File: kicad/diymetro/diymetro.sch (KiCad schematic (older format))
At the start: 45 parts, among them J1 Conn_02x08_Top_Bottom, J10 ReverseSwitch, J11 Conn_01x04, J12 +5V, J2 CLKGATE_Pots, J3 Gate_Pots, J4 CV_Pots, J5 CLKOUT, J6 GATEOUT, J7 CVOUT, J8 LEDs, J9 Conn_01x04, U1 74HC4051, U2 74HC4051, U3 74LS594, U4 74LS165

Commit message: Update schematic a bit.
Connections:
- net labels added: CLK165, SHLD
- net labels removed: CE, CP
- wire segments 155 -> 156
- no-connect marks 24 -> 23
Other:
- note added: "Wiring Notes:\n\n* Connect pots to +5V and GND. \n* Pot tapers to the CV + Gate connectors.\n* Pots are 10k.\n* Connect jacks to GND and connectors.\n* Connect switches to +5V and connectors.\n* LED cathodes to GND and LED connector.\n* Play with 74LS594 resistors to match your LEDs."
- moved on the sheet: J1, R12, R13, R14, R15, R16, R17, R18, R19

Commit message: Work on clock input.
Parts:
- added J13: CLOCK_INPUT, symbol Connector:AudioJack2_SwitchT
- added Q1: PN2222A, Package_TO_SOT_THT:TO-92_Inline, symbol Transistor_BJT:PN2222A
- added R20: 1M, Resistor_THT:R_Axial_DIN0207_L6.3mm_D2.5mm_P7.62mm_Horizontal, symbol Device:R
- added R21: 100K, Resistor_THT:R_Axial_DIN0207_L6.3mm_D2.5mm_P7.62mm_Horizontal, symbol Device:R
- added R22: 10K, Resistor_THT:R_Axial_DIN0207_L6.3mm_D2.5mm_P7.62mm_Horizontal, symbol Device:R
- J10: value ReverseSwitch -> MainSW
- J5: value CLKOUT -> GATEOUT
- J6: value GATEOUT -> CLKOUT
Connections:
- net labels added: CINSW, CLK_IN
- wire segments 156 -> 172
- no-connect marks 23 -> 21
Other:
- moved on the sheet: C1, C2, C3, C4, C5, D1, D2, J1, R1, R10, R11, R3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

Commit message: Update code and schematics for clock and reset input.
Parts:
- removed J10: MainSW, Connector_PinHeader_2.54mm:PinHeader_1x01_P2.54mm_Vertical, symbol Connector:Conn_01x01_Female
- added J10: MAINSW, Connector_PinHeader_2.54mm:PinHeader_1x01_P2.54mm_Vertical, symbol Connector_Generic:Conn_01x01
- added J14: RESET_INPUT, symbol Connector:AudioJack2_SwitchT
- added Q2: PN2222A, Package_TO_SOT_THT:TO-92_Inline, symbol Transistor_BJT:PN2222A
- added R23: 100K, Resistor_THT:R_Axial_DIN0207_L6.3mm_D2.5mm_P7.62mm_Horizontal, symbol Device:R
- added R24: 10K, Resistor_THT:R_Axial_DIN0207_L6.3mm_D2.5mm_P7.62mm_Horizontal, symbol Device:R
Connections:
- net labels added: RST_IN
- net labels removed: CLK165
- wire segments 172 -> 180
- no-connect marks 21 -> 22
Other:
- moved on the sheet: C1, C2, C3, C4, C5, C6, D1, D2, D3, J1, J13, Q1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

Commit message: New schematics and boards.
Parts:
- removed A1: Arduino_Nano_v3.x, Module:Arduino_Nano, symbol MCU_Module:Arduino_Nano_v3.x
- removed C1, C3: 220n, Capacitor_THT:C_Rect_L7.0mm_W3.5mm_P2.50mm_P5.00mm, symbol Device:C
- removed C2, C4: 100n, Capacitor_THT:C_Axial_L3.8mm_D2.6mm_P7.50mm_Horizontal, symbol Device:C
- removed D3: D, Diode_THT:D_DO-15_P10.16mm_Horizontal, symbol Device:D
- removed J1: Conn_02x08_Top_Bottom, Connector_PinHeader_2.54mm:PinHeader_2x08_P2.54mm_Vertical, symbol Connector_Generic:Conn_02x08_Odd_Even
- removed J10: MAINSW, Connector_PinHeader_2.54mm:PinHeader_1x01_P2.54mm_Vertical, symbol Connector_Generic:Conn_01x01
- removed J11, J9: Conn_01x04, Connector_PinHeader_2.54mm:PinHeader_1x04_P2.54mm_Vertical, symbol Connector_Generic:Conn_01x04
- removed J12: +5V, Connector_PinHeader_2.54mm:PinHeader_1x01_P2.54mm_Vertical, symbol Connector_Generic:Conn_01x01
- removed J13: CLOCK_INPUT, symbol Connector:AudioJack2_SwitchT
- removed J14: RESET_INPUT, symbol Connector:AudioJack2_SwitchT
- removed J2: CLKGATE_Pots, Connector_PinHeader_2.54mm:PinHeader_1x02_P2.54mm_Vertical, symbol Connector_Generic:Conn_01x02
- removed J3: Gate_Pots, Connector_PinHeader_2.54mm:PinHeader_1x08_P2.54mm_Vertical, symbol Connector_Generic:Conn_01x08
- removed J4: CV_Pots, Connector_PinHeader_2.54mm:PinHeader_1x08_P2.54mm_Vertical, symbol Connector_Generic:Conn_01x08
- removed J5: GATEOUT, Connector_PinHeader_2.54mm:PinHeader_1x01_P2.54mm_Vertical, symbol Connector_Generic:Conn_01x01
- removed J6: CLKOUT, Connector_PinHeader_2.54mm:PinHeader_1x01_P2.54mm_Vertical, symbol Connector_Generic:Conn_01x01
- removed J7: CVOUT, Connector_PinHeader_2.54mm:PinHeader_1x01_P2.54mm_Vertical, symbol Connector_Generic:Conn_01x01
- removed J8: LEDs, Connector_PinHeader_2.54mm:PinHeader_1x08_P2.54mm_Vertical, symbol Connector_Generic:Conn_01x08
- removed R10, R11, R8, R9: 220, Resistor_THT:R_Axial_DIN0207_L6.3mm_D2.5mm_P7.62mm_Horizontal, symbol Device:R
- removed R12, R13, R14, R15, R16, R17, R18, R19, R22, R24: 10K, Resistor_THT:R_Axial_DIN0207_L6.3mm_D2.5mm_P7.62mm_Horizontal, symbol Device:R
- removed R20: 1M, Resistor_THT:R_Axial_DIN0207_L6.3mm_D2.5mm_P7.62mm_Horizontal, symbol Device:R
- removed R21, R23: 100K, Resistor_THT:R_Axial_DIN0207_L6.3mm_D2.5mm_P7.62mm_Horizontal, symbol Device:R
- removed U1, U2: 74HC4051, Package_DIP:DIP-16_W7.62mm, symbol 74xx:74HC4051
- removed U3: 74LS594, Package_DIP:DIP-16_W7.62mm, symbol 74xx_IEEE:74LS594
- removed U4: 74LS165, Package_DIP:DIP-16_W7.62mm, symbol 74xx:74LS165
- added C7, C8: 100n, Capacitor_SMD:C_1206_3216Metric, symbol Device:C
- added D14: LED, LED_THT:LED_D3.0mm, symbol Device:LED
- added J1, J2, J3, J4, J6: AudioJack2_SwitchT, Connector_Audio:Jack_3.5mm_QingPu_WQP-PJ398SM_Vertical_CircularHoles, symbol Connector:AudioJack2_SwitchT
- added J5: Conn_02x08_Top_Bottom, Connector_IDC:IDC-Header_2x08_P2.54mm_Vertical, symbol Connector_Generic:Conn_02x08_Odd_Even
- added J7: ICSP, Connector_PinHeader_2.54mm:PinHeader_2x03_P2.54mm_Vertical, symbol Connector_Generic:Conn_02x03_Odd_Even
- added J8: SER, Connector_PinHeader_2.54mm:PinHeader_1x02_P2.54mm_Vertical, symbol Connector:Conn_01x02_Male
- added R45: 10k, Resistor_SMD:R_1206_3216Metric, symbol Device:R
- added R46: 1K, Resistor_SMD:R_1206_3216Metric, symbol Device:R
- added RV1, RV2: R_POT, Potentiometer_THT:Potentiometer_Alps_RK09K_Single_Vertical, symbol Device:R_POT
- added SW10: SW_Push, Button_Switch_THT:SW_PUSH_6mm, symbol Switch:SW_Push
- added U5: ATmega328P-PU, Package_DIP:DIP-28_W7.62mm, symbol MCU_Microchip_ATmega:ATmega328P-PU
- added Y1: Crystal, Crystal:Crystal_HC49-4H_Vertical, symbol Device:Crystal
- C5, C6: value 100n -> 22p; footprint Capacitor_THT:C_Axial_L3.8mm_D2.6mm_P7.50mm_Horizontal -> Capacitor_SMD:C_1206_3216Metric
- D1, D2: footprint Diode_THT:D_DO-15_P10.16mm_Horizontal -> Diode_SMD:D_1206_3216Metric
- Q1, Q2: footprint Package_TO_SOT_THT:TO-92_Inline -> Package_TO_SOT_SMD:SOT-23
- R1, R2, R3: footprint Resistor_THT:R_Axial_DIN0207_L6.3mm_D2.5mm_P7.62mm_Horizontal -> Resistor_SMD:R_1206_3216Metric
- R4, R7: value 220 -> 100K; footprint Resistor_THT:R_Axial_DIN0207_L6.3mm_D2.5mm_P7.62mm_Horizontal -> Resistor_SMD:R_1206_3216Metric
- R5: value 220 -> 10K; footprint Resistor_THT:R_Axial_DIN0207_L6.3mm_D2.5mm_P7.62mm_Horizontal -> Resistor_SMD:R_1206_3216Metric
- R6: value 220 -> 1M; footprint Resistor_THT:R_Axial_DIN0207_L6.3mm_D2.5mm_P7.62mm_Horizontal -> Resistor_SMD:R_1206_3216Metric
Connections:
- net labels added: AP_CLK_IN, AP_CLK_OUT, AP_GATE_OUT, AP_RST_IN, ICSP_MISO, ICSP_MOSI, ICSP_RST, ICSP_SCK, PIN_CLKPOT, PIN_CVOUT, PIN_GATEOUT, PIN_GATEPOT, RA, SA
- net labels removed: CLK_IN, QH, RST_IN, SHLD
- wire segments 180 -> 84
- no-connect marks 22 -> 14
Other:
- note removed: "Wiring Notes:\n\n* Connect pots to +5V and GND. \n* Pot tapers to the CV + Gate connectors.\n* Pots are 10k.\n* Connect jacks to GND and connectors.\n* Connect switches to +5V and connectors.\n* LED cathodes to GND and LED connector.\n* Play with 74LS594 resistors to match your LEDs."

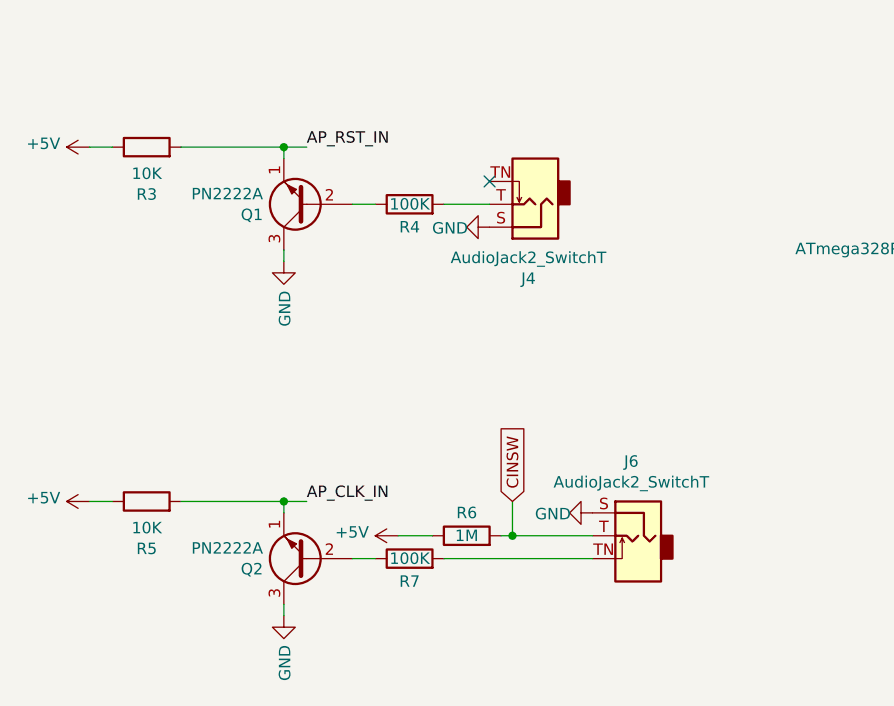
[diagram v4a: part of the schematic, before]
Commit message: Fix 74hc595 OE pin, Fix MBT2222A symbol + footprint, Fix clock-in jack connections.
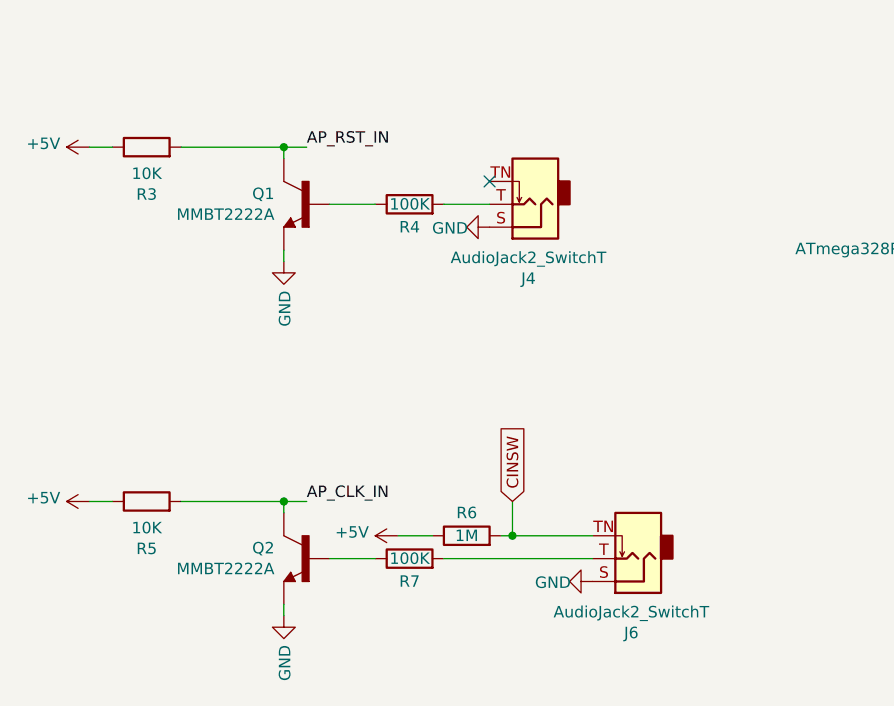
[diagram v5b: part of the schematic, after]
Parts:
- removed Q1, Q2: PN2222A, Package_TO_SOT_SMD:SOT-23, symbol Transistor_BJT:PN2222A
- added Q1, Q2: MMBT2222A, MMBT2222A:SOT23, symbol MMBT2222A:MMBT2222A
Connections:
- net AP_CLK_IN: now also Q2.3 (C)
- net AP_RST_IN: now also Q1.3 (C)
- net CINSW: now also J6.TN; no longer J6.T
- net GND: now also Q1.2 (E), Q2.2 (E)
- net at R7.1: now also Q2.1 (B)
- net at R7.2: now also J6.T; no longer J6.TN
- net at R4.1: now also Q1.1 (B)
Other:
- moved on the sheet: J6
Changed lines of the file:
@@
 	8500 3850 8550 3850
-$Comp
-L Transistor_BJT:PN2222A Q?
-U 1 1 5D188326
-P 2400 6050
-AR Path="/5CAA6291/5D188326" Ref="Q?"  Part="1"
-AR Path="/5D188326" Ref="Q2"  Part="1"
-F 0 "Q2" H 2591 6096 50  0000 L CNN
-F 1 "PN2222A" H 2591 6005 50  0000 L CNN
-F 2 "Package_TO_SOT_SMD:SOT-23" H 2600 5975 50  0001 L CIN
-F 3 "http://www.fairchildsemi.com/ds/PN/PN2222A.pdf" H 2400 6050 50  0001 L CNN
-	1    2400 6050
-	-1   0    0    1
-$EndComp
 $Comp
 L Device:R R?
@@
 	0    -1   -1   0
 $EndComp
-Wire Wire Line
-	2600 6050 2700 6050
 $Comp
 L power:GND #PWR?
@@
 Wire Wire Line
 	3250 5950 3300 5950
-Connection ~ 3300 5950
 Wire Wire Line
 	3300 5800 3300 5950
@@
 	2300 6300 2300 6250
 $Comp
-L Transistor_BJT:PN2222A Q?
-U 1 1 5D188368
-P 2400 4500
-AR Path="/5CAA6291/5D188368" Ref="Q?"  Part="1"
-AR Path="/5D188368" Ref="Q1"  Part="1"
-F 0 "Q1" H 2591 4546 50  0000 L CNN
-F 1 "PN2222A" H 2591 4455 50  0000 L CNN
-F 2 "Package_TO_SOT_SMD:SOT-23" H 2600 4425 50  0001 L CIN
-F 3 "http://www.fairchildsemi.com/ds/PN/PN2222A.pdf" H 2400 4500 50  0001 L CNN
-	1    2400 4500
-	-1   0    0    1
-$EndComp
-$Comp
 L Device:R R?
 U 1 1 5D18836F
@@
 	0    -1   -1   0
 $EndComp
-Wire Wire Line
-	2600 4500 2700 4500
 $Comp
 L power:GND #PWR?
@@
 L Connector:AudioJack2_SwitchT J?
 U 1 1 5D194F65
-P 3850 5950
+P 3850 6050
 AR Path="/5CA98B27/5D194F65" Ref="J?"  Part="1"
 AR Path="/5D194F65" Ref="J6"  Part="1"
-F 0 "J6" H 3880 6275 50  0000 C CNN
-F 1 "AudioJack2_SwitchT" H 3880 6184 50  0000 C CNN
-F 2 "Connector_Audio:Jack_3.5mm_QingPu_WQP-PJ398SM_Vertical_CircularHoles" H 3850 5950 50  0001 C CNN
-F 3 "~" H 3850 5950 50  0001 C CNN
-	1    3850 5950
-	-1   0    0    -1
+F 0 "J6" H 3880 6375 50  0000 C CNN
+F 1 "AudioJack2_SwitchT" H 3880 6284 50  0000 C CNN
+F 2 "Connector_Audio:Jack_3.5mm_QingPu_WQP-PJ398SM_Vertical_CircularHoles" H 3850 6050 50  0001 C CNN
+F 3 "~" H 3850 6050 50  0001 C CNN
+	1    3850 6050
+	-1   0    0    1
 $EndComp
 $Comp
@@
 Wire Wire Line
 	3000 6050 3650 6050
-Wire Wire Line
-	3300 5950 3650 5950
 $Comp
 L power:GND #PWR?
 U 1 1 5D1BFD84
-P 3650 5850
+P 3650 6150
 AR Path="/5CAA6291/5D1BFD84" Ref="#PWR?"  Part="1"
 AR Path="/5D1BFD84" Ref="#PWR031"  Part="1"
-F 0 "#PWR031" H 3650 5600 50  0001 C CNN
-F 1 "GND" V 3655 5677 50  0000 C CNN
-F 2 "" H 3650 5850 50  0001 C CNN
-F 3 "" H 3650 5850 50  0001 C CNN
-	1    3650 5850
+F 0 "#PWR031" H 3650 5900 50  0001 C CNN
+F 1 "GND" V 3655 5977 50  0000 C CNN
+F 2 "" H 3650 6150 50  0001 C CNN
+F 3 "" H 3650 6150 50  0001 C CNN
+	1    3650 6150
 	0    1    1    0
 $EndComp
@@
 	0    -1   -1   0
 $EndComp
+Wire Wire Line
+	2500 4500 2700 4500
+$Comp
+L MMBT2222A:MMBT2222A Q2
+U 1 1 5D860213
+P 2400 6050
+F 0 "Q2" H 2541 6096 50  0000 L CNN
+F 1 "MMBT2222A" H 2541 6005 50  0000 L CNN
+F 2 "MMBT2222A:SOT23" H 2400 6050 50  0001 L BNN
+F 3 "Unavailable" H 2400 6050 50  0001 L BNN
+F 4 "Fairchild Semiconductor" H 2400 6050 50  0001 L BNN "Field4"
+F 5 "MMBT2222 Series 40 V CE Breakdown 1 A NPN General Purpose Amplifier - SOT-23" H 2400 6050 50  0001 L BNN "Field5"
+F 6 "None" H 2400 6050 50  0001 L BNN "Field6"
+F 7 "SOT-23 Fairchild Semiconductor" H 2400 6050 50  0001 L BNN "Field7"
+F 8 "MMBT2222A." H 2400 6050 50  0001 L BNN "Field8"
+	1    2400 6050
+	-1   0    0    -1
+$EndComp
+Wire Wire Line
+	2500 6050 2700 6050
+$Comp
+L MMBT2222A:MMBT2222A Q1
+U 1 1 5D862FDE
+P 2400 4500
+F 0 "Q1" H 2541 4546 50  0000 L CNN
+F 1 "MMBT2222A" H 2541 4455 50  0000 L CNN
+F 2 "MMBT2222A:SOT23" H 2400 4500 50  0001 L BNN
+F 3 "Unavailable" H 2400 4500 50  0001 L BNN
+F 4 "Fairchild Semiconductor" H 2400 4500 50  0001 L BNN "Field4"
+F 5 "MMBT2222 Series 40 V CE Breakdown 1 A NPN General Purpose Amplifier - SOT-23" H 2400 4500 50  0001 L BNN "Field5"
+F 6 "None" H 2400 4500 50  0001 L BNN "Field6"
+F 7 "SOT-23 Fairchild Semiconductor" H 2400 4500 50  0001 L BNN "Field7"
+F 8 "MMBT2222A." H 2400 4500 50  0001 L BNN "Field8"
+	1    2400 4500
+	-1   0    0    -1
+$EndComp
+Connection ~ 3300 5950
+Wire Wire Line
+	3300 5950 3650 5950
 $EndSCHEMATC

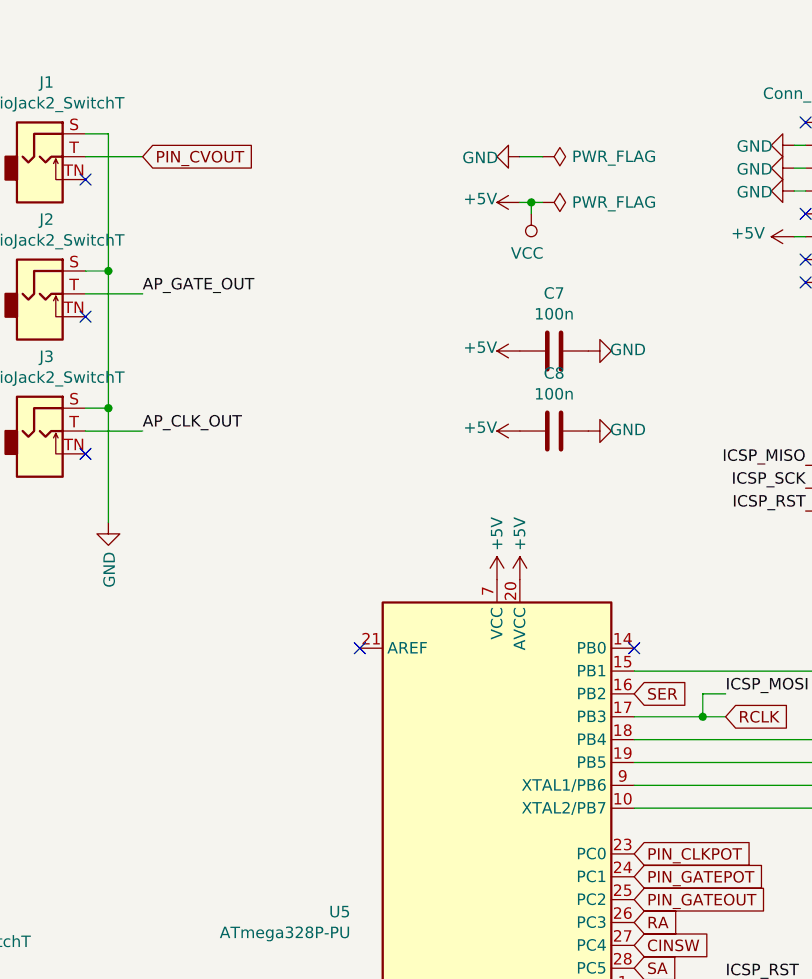
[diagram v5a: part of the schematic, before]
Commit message: Add missing C9
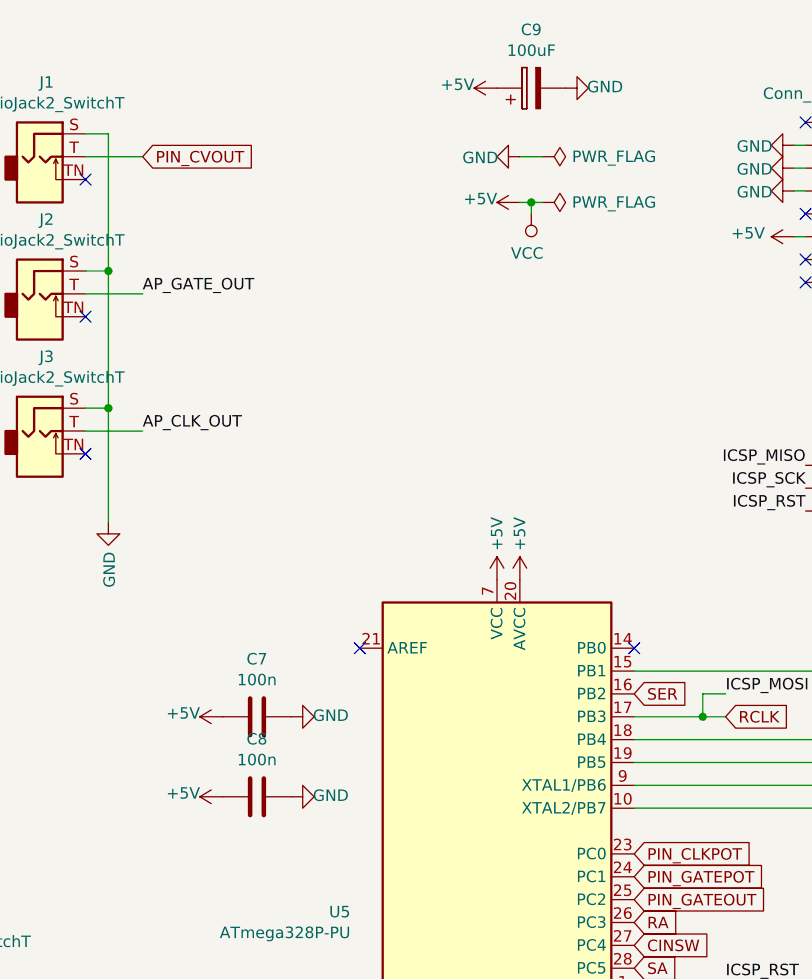
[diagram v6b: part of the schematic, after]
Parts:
- added C9: 100uF, symbol Device:CP
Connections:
- net +5V: now also C9.1
- net GND: now also C9.2
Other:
- moved on the sheet: C7, C8
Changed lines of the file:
@@
 L power:+5V #PWR?
 U 1 1 5D744A36
-P 5850 2150
+P 4550 3750
 AR Path="/5CAA6291/5D744A36" Ref="#PWR?"  Part="1"
 AR Path="/5D744A36" Ref="#PWR08"  Part="1"
-F 0 "#PWR08" H 5850 2000 50  0001 C CNN
-F 1 "+5V" V 5865 2323 50  0000 C CNN
-F 2 "" H 5850 2150 50  0001 C CNN
-F 3 "" H 5850 2150 50  0001 C CNN
-	1    5850 2150
+F 0 "#PWR08" H 4550 3600 50  0001 C CNN
+F 1 "+5V" V 4565 3923 50  0000 C CNN
+F 2 "" H 4550 3750 50  0001 C CNN
+F 3 "" H 4550 3750 50  0001 C CNN
+	1    4550 3750
 	0    -1   -1   0
 $EndComp
@@
 L Device:C C7
 U 1 1 5D744A7B
-P 6000 2150
-F 0 "C7" V 5748 2150 50  0000 C CNN
-F 1 "100n" V 5839 2150 50  0000 C CNN
-F 2 "Capacitor_SMD:C_1206_3216Metric" H 6038 2000 50  0001 C CNN
-F 3 "~" H 6000 2150 50  0001 C CNN
-	1    6000 2150
+P 4700 3750
+F 0 "C7" V 4448 3750 50  0000 C CNN
+F 1 "100n" V 4539 3750 50  0000 C CNN
+F 2 "Capacitor_SMD:C_1206_3216Metric" H 4738 3600 50  0001 C CNN
+F 3 "~" H 4700 3750 50  0001 C CNN
+	1    4700 3750
 	0    1    1    0
 $EndComp
@@
 L power:GND #PWR?
 U 1 1 5D744B09
-P 6150 2150
+P 4850 3750
 AR Path="/5CAA6291/5D744B09" Ref="#PWR?"  Part="1"
 AR Path="/5D744B09" Ref="#PWR015"  Part="1"
-F 0 "#PWR015" H 6150 1900 50  0001 C CNN
-F 1 "GND" V 6155 1977 50  0000 C CNN
-F 2 "" H 6150 2150 50  0001 C CNN
-F 3 "" H 6150 2150 50  0001 C CNN
-	1    6150 2150
+F 0 "#PWR015" H 4850 3500 50  0001 C CNN
+F 1 "GND" V 4855 3577 50  0000 C CNN
+F 2 "" H 4850 3750 50  0001 C CNN
+F 3 "" H 4850 3750 50  0001 C CNN
+	1    4850 3750
 	0    -1   -1   0
 $EndComp
@@
 L power:+5V #PWR?
 U 1 1 5D744CC7
-P 5850 2500
+P 4550 4100
 AR Path="/5CAA6291/5D744CC7" Ref="#PWR?"  Part="1"
 AR Path="/5D744CC7" Ref="#PWR029"  Part="1"
-F 0 "#PWR029" H 5850 2350 50  0001 C CNN
-F 1 "+5V" V 5865 2673 50  0000 C CNN
-F 2 "" H 5850 2500 50  0001 C CNN
-F 3 "" H 5850 2500 50  0001 C CNN
-	1    5850 2500
+F 0 "#PWR029" H 4550 3950 50  0001 C CNN
+F 1 "+5V" V 4565 4273 50  0000 C CNN
+F 2 "" H 4550 4100 50  0001 C CNN
+F 3 "" H 4550 4100 50  0001 C CNN
+	1    4550 4100
 	0    -1   -1   0
 $EndComp
@@
 L Device:C C8
 U 1 1 5D744CCD
-P 6000 2500
-F 0 "C8" V 5748 2500 50  0000 C CNN
-F 1 "100n" V 5839 2500 50  0000 C CNN
-F 2 "Capacitor_SMD:C_1206_3216Metric" H 6038 2350 50  0001 C CNN
-F 3 "~" H 6000 2500 50  0001 C CNN
-	1    6000 2500
+P 4700 4100
+F 0 "C8" V 4448 4100 50  0000 C CNN
+F 1 "100n" V 4539 4100 50  0000 C CNN
+F 2 "Capacitor_SMD:C_1206_3216Metric" H 4738 3950 50  0001 C CNN
+F 3 "~" H 4700 4100 50  0001 C CNN
+	1    4700 4100
 	0    1    1    0
 $EndComp
@@
 L power:GND #PWR?
 U 1 1 5D744CD4
-P 6150 2500
+P 4850 4100
 AR Path="/5CAA6291/5D744CD4" Ref="#PWR?"  Part="1"
 AR Path="/5D744CD4" Ref="#PWR034"  Part="1"
-F 0 "#PWR034" H 6150 2250 50  0001 C CNN
-F 1 "GND" V 6155 2327 50  0000 C CNN
-F 2 "" H 6150 2500 50  0001 C CNN
-F 3 "" H 6150 2500 50  0001 C CNN
-	1    6150 2500
+F 0 "#PWR034" H 4850 3850 50  0001 C CNN
+F 1 "GND" V 4855 3927 50  0000 C CNN
+F 2 "" H 4850 4100 50  0001 C CNN
+F 3 "" H 4850 4100 50  0001 C CNN
+	1    4850 4100
 	0    -1   -1   0
 $EndComp
@@
 Wire Wire Line
 	3300 5950 3650 5950
+$Comp
+L Device:CP C9
+U 1 1 5D85797C
+P 5900 1000
+F 0 "C9" V 6155 1000 50  0000 C CNN
+F 1 "100uF" V 6064 1000 50  0000 C CNN
+F 2 "" H 5938 850 50  0001 C CNN
+F 3 "~" H 5900 1000 50  0001 C CNN
+	1    5900 1000
+	0    -1   -1   0
+$EndComp
+$Comp
+L power:+5V #PWR?
+U 1 1 5D8588F1
+P 5750 1000
+AR Path="/5CAA6291/5D8588F1" Ref="#PWR?"  Part="1"
+AR Path="/5D8588F1" Ref="#PWR035"  Part="1"
+F 0 "#PWR035" H 5750 850 50  0001 C CNN
+F 1 "+5V" V 5765 1173 50  0000 C CNN
+F 2 "" H 5750 1000 50  0001 C CNN
+F 3 "" H 5750 1000 50  0001 C CNN
+	1    5750 1000
+	0    -1   -1   0
+$EndComp
+$Comp
+L power:GND #PWR?
+U 1 1 5D85897C
+P 6050 1000
+AR Path="/5CAA6291/5D85897C" Ref="#PWR?"  Part="1"
+AR Path="/5D85897C" Ref="#PWR036"  Part="1"
+F 0 "#PWR036" H 6050 750 50  0001 C CNN
+F 1 "GND" V 6055 827 50  0000 C CNN
+F 2 "" H 6050 1000 50  0001 C CNN
+F 3 "" H 6050 1000 50  0001 C CNN
+	1    6050 1000
+	0    -1   -1   0
+$EndComp
 $EndSCHEMATC

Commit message: Add missing footprint for C9
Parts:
- C9: footprint (none) -> Tomarus:GenericCap
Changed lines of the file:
@@
 F 0 "C9" V 6155 1000 50  0000 C CNN
 F 1 "100uF" V 6064 1000 50  0000 C CNN
-F 2 "" H 5938 850 50  0001 C CNN
+F 2 "Tomarus:GenericCap" H 5938 850 50  0001 C CNN
 F 3 "~" H 5900 1000 50  0001 C CNN
 	1    5900 1000
